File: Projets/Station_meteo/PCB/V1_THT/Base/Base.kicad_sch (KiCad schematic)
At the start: 9 parts, among them J13 JST_PH_4P

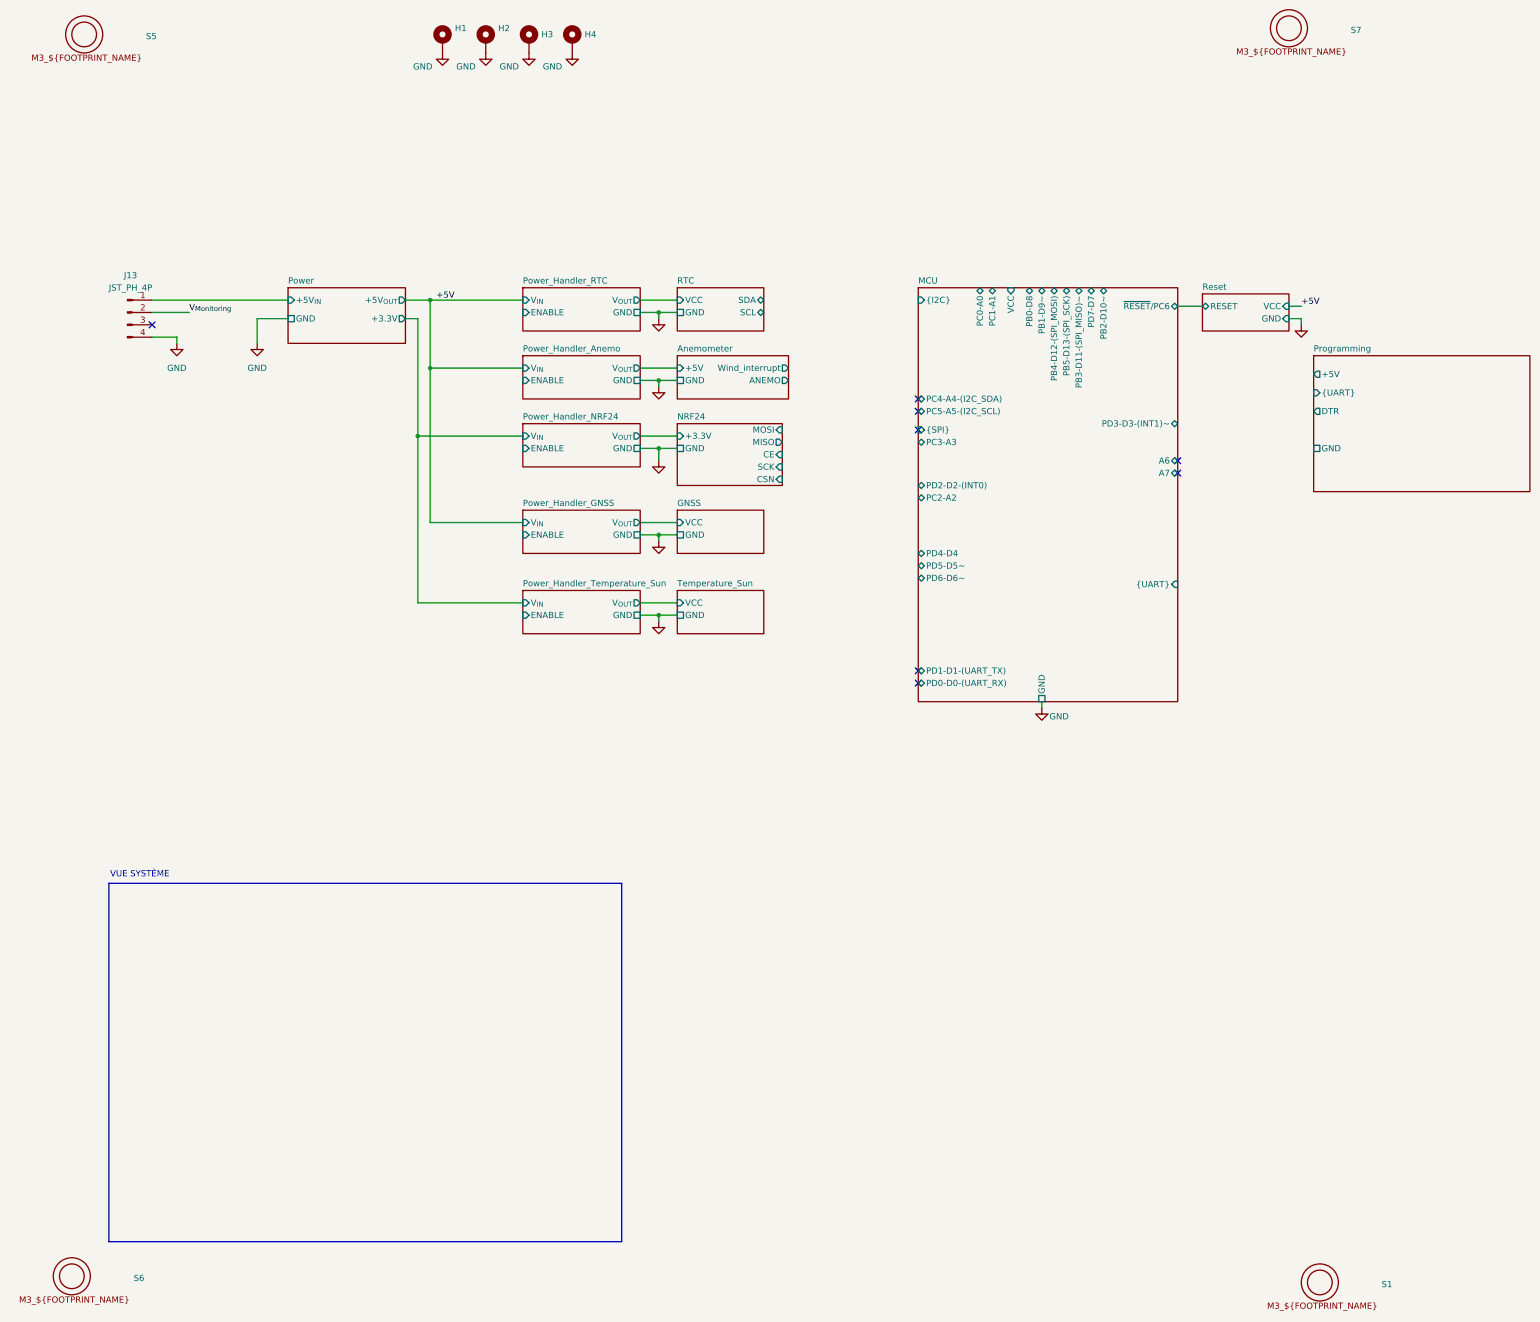
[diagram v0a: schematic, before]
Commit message: Update
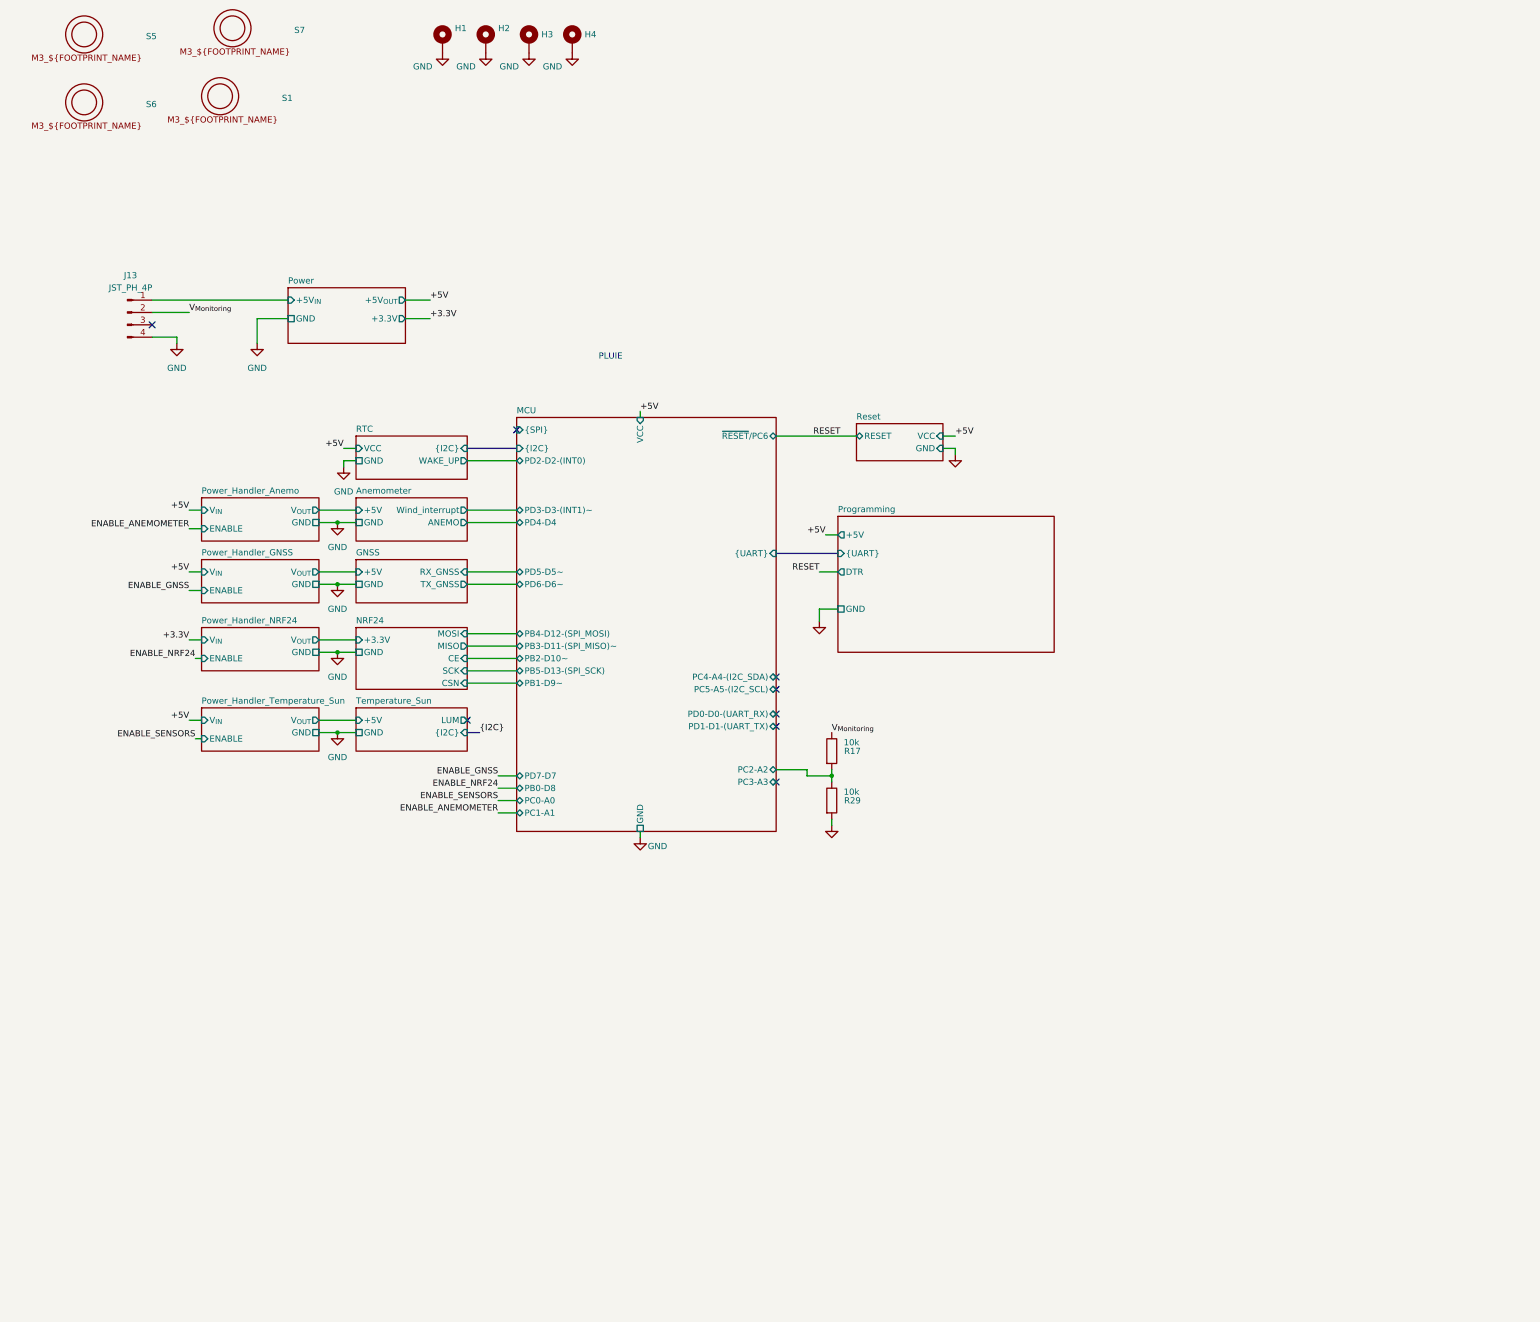
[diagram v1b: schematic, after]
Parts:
- added R17, R29: 10k, Resistor_THT:R_Axial_DIN0207_L6.3mm_D2.5mm_P7.62mm_Horizontal, symbol CREPP_Resistors:Resistor_THT_250mW (standard)
- J13: now left out of the parts list
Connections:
- net GND: now also R29.2
- net MCU/PC2-A2: now also R17.2, R29.1
- net V_{Monitoring}: now also R17.1
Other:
- removed sheet Power_Handler_RTC
- sheet GNSS ports: added +5V, RX_GNSS, TX_GNSS; removed VCC
- sheet MCU ports: added none; removed A6, A7
- sheet RTC ports: added WAKE_UP, {I2C}; removed SCL, SDA
- sheet Temperature_Sun ports: added +5V, LUM, {I2C}; removed VCC
- note added: "PLUIE"
- note removed: "VUE SYSTÈME"
- moved on the sheet: S1, S6, S7
